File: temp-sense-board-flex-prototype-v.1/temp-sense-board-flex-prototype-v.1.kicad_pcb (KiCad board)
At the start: 2 copper layers, 134.7 x 89.8 mm, 30 parts, among them J2 FH34SRJ-12S-0.5SH(50), J3 FH12-12S-1SH(55), J4 1-84953-2, U1 TMP1075D, U2 TMP1075D, U3 TMP1075D

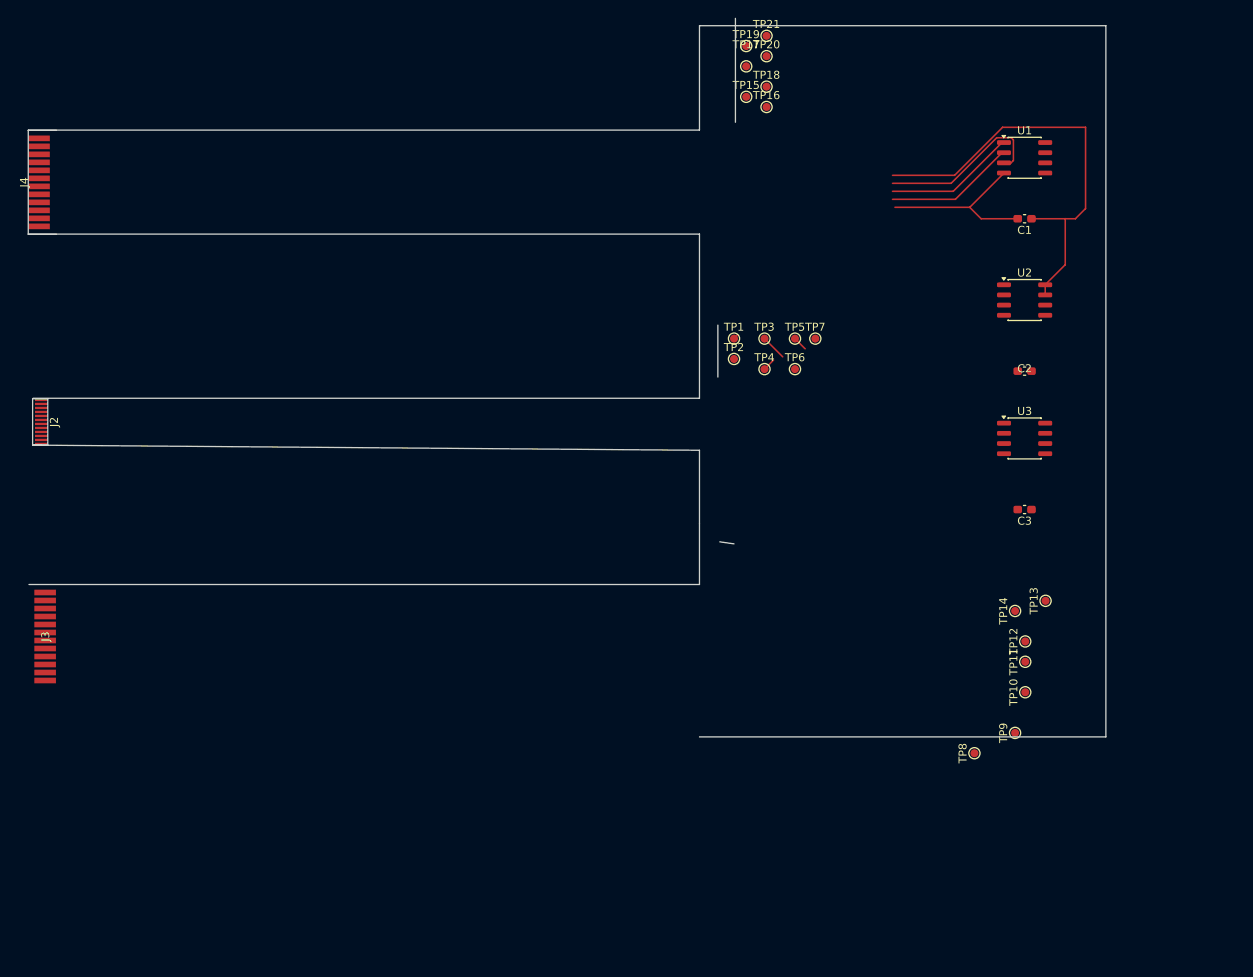
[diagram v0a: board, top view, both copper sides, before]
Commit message: outline added and layout started
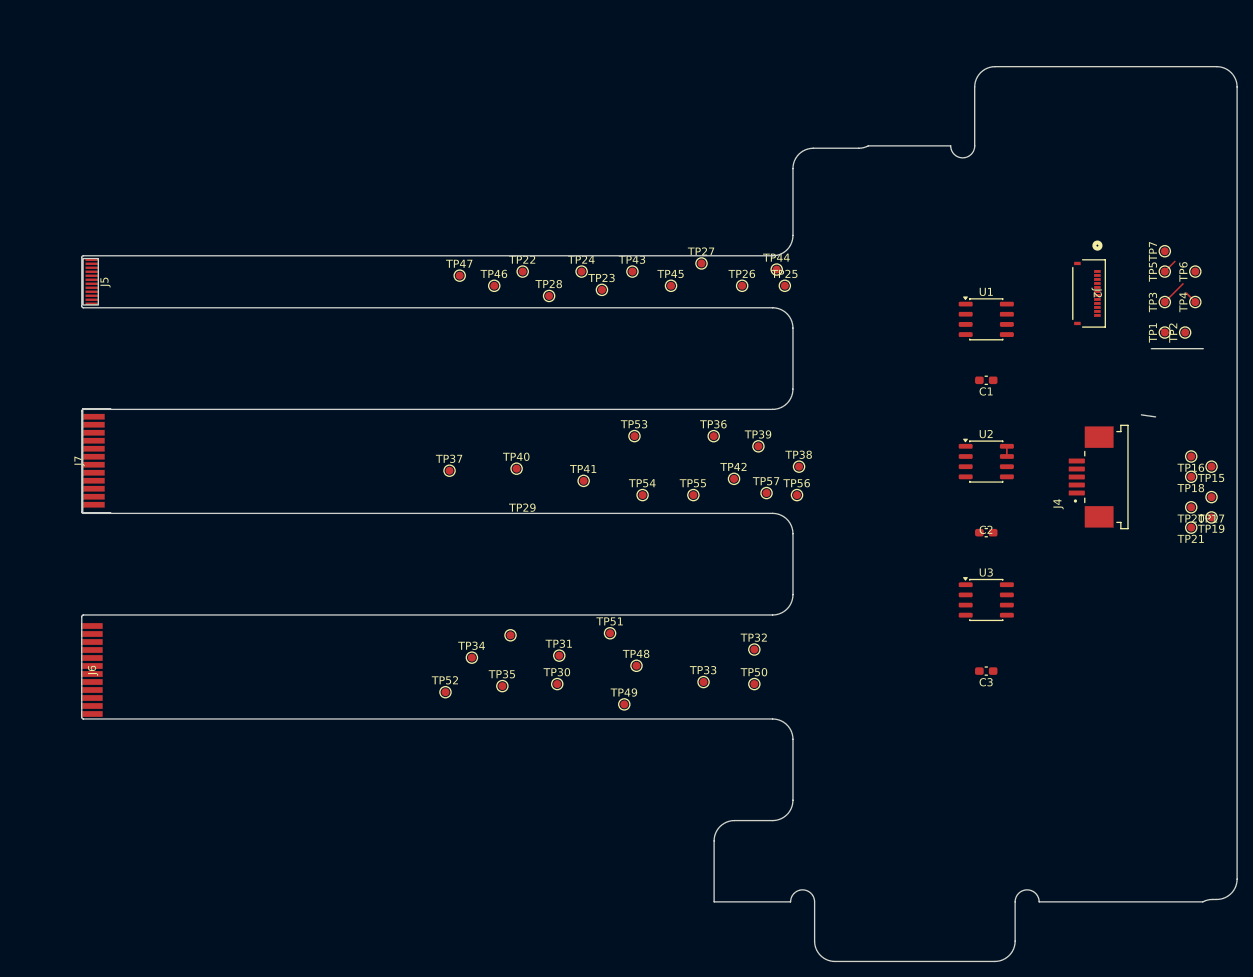
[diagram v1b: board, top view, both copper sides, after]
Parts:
- removed J3: FH12-12S-1SH(55), formula_slug_footprint_library:FPC-12PIN-CABLE-1mm-0.65mm
- removed TP10, TP11, TP12, TP13, TP14, TP8, TP9: TestPoint, TestPoint:TestPoint_Pad_D1.0mm
- added J5: FH34SRJ-12S-0.5SH(50), formula_slug_footprint_library:FPC_12-CABLE-0.5mm-0.3mm, F.Cu at (51.9, 57.4)
- added J6: FH12-12S-1SH(55), formula_slug_footprint_library:FPC-12PIN-CABLE-1mm-0.65mm, F.Cu at (49.7, 105.9)
- added J7: 1-84953-2, formula_slug_footprint_library:FPC-12PIN-CABLE-1mm-0.71mm, F.Cu at (49.9, 79.8)
- added TP22: TestPoint, TestPoint:TestPoint_Pad_D1.0mm, F.Cu at (104.9, 56.1)
- added TP23: TestPoint, TestPoint:TestPoint_Pad_D1.0mm, F.Cu at (114.8, 58.4)
- added TP24: TestPoint, TestPoint:TestPoint_Pad_D1.0mm, F.Cu at (112.3, 56.1)
- added TP25: TestPoint, TestPoint:TestPoint_Pad_D1.0mm, F.Cu at (137.7, 57.9)
- added TP26: TestPoint, TestPoint:TestPoint_Pad_D1.0mm, F.Cu at (132.3, 57.9)
- added TP27: TestPoint, TestPoint:TestPoint_Pad_D1.0mm, F.Cu at (127.3, 55.1)
- added TP28: TestPoint, TestPoint:TestPoint_Pad_D1.0mm, F.Cu at (108.2, 59.2)
- added TP29: TestPoint, TestPoint:TestPoint_Pad_D1.0mm, F.Cu at (103.4, 101.6)
- added TP30: TestPoint, TestPoint:TestPoint_Pad_D1.0mm, F.Cu at (109.2, 107.7)
- added TP31: TestPoint, TestPoint:TestPoint_Pad_D1.0mm, F.Cu at (109.5, 104.1)
- added TP32: TestPoint, TestPoint:TestPoint_Pad_D1.0mm, F.Cu at (133.9, 103.4)
- added TP33: TestPoint, TestPoint:TestPoint_Pad_D1.0mm, F.Cu at (127.5, 107.4)
- added TP34: TestPoint, TestPoint:TestPoint_Pad_D1.0mm, F.Cu at (98.6, 104.4)
- added TP35: TestPoint, TestPoint:TestPoint_Pad_D1.0mm, F.Cu at (102.4, 108.0)
- added TP36: TestPoint, TestPoint:TestPoint_Pad_D1.0mm, F.Cu at (128.8, 76.7)
- added TP37: TestPoint, TestPoint:TestPoint_Pad_D1.0mm, F.Cu at (95.8, 81.0)
- added TP38: TestPoint, TestPoint:TestPoint_Pad_D1.0mm, F.Cu at (139.4, 80.5)
- added TP39: TestPoint, TestPoint:TestPoint_Pad_D1.0mm, F.Cu at (134.4, 78.0)
- added TP40: TestPoint, TestPoint:TestPoint_Pad_D1.0mm, F.Cu at (104.1, 80.8)
- added TP41: TestPoint, TestPoint:TestPoint_Pad_D1.0mm, F.Cu at (112.5, 82.3)
- added TP42: TestPoint, TestPoint:TestPoint_Pad_D1.0mm, F.Cu at (131.3, 82.0)
- added TP43: TestPoint, TestPoint:TestPoint_Pad_D1.0mm, F.Cu at (118.6, 56.1)
- added TP44: TestPoint, TestPoint:TestPoint_Pad_D1.0mm, F.Cu at (136.7, 55.9)
- added TP45: TestPoint, TestPoint:TestPoint_Pad_D1.0mm, F.Cu at (123.4, 57.9)
- added TP46: TestPoint, TestPoint:TestPoint_Pad_D1.0mm, F.Cu at (101.3, 57.9)
- added TP47: TestPoint, TestPoint:TestPoint_Pad_D1.0mm, F.Cu at (97.0, 56.6)
- added TP48: TestPoint, TestPoint:TestPoint_Pad_D1.0mm, F.Cu at (119.1, 105.4)
- added TP49: TestPoint, TestPoint:TestPoint_Pad_D1.0mm, F.Cu at (117.6, 110.2)
- added TP50: TestPoint, TestPoint:TestPoint_Pad_D1.0mm, F.Cu at (133.9, 107.7)
- added TP51: TestPoint, TestPoint:TestPoint_Pad_D1.0mm, F.Cu at (115.8, 101.3)
- added TP52: TestPoint, TestPoint:TestPoint_Pad_D1.0mm, F.Cu at (95.2, 108.7)
- added TP53: TestPoint, TestPoint:TestPoint_Pad_D1.0mm, F.Cu at (118.9, 76.7)
- added TP54: TestPoint, TestPoint:TestPoint_Pad_D1.0mm, F.Cu at (119.9, 84.1)
- added TP55: TestPoint, TestPoint:TestPoint_Pad_D1.0mm, F.Cu at (126.2, 84.1)
- added TP56: TestPoint, TestPoint:TestPoint_Pad_D1.0mm, F.Cu at (139.2, 84.1)
- added TP57: TestPoint, TestPoint:TestPoint_Pad_D1.0mm, F.Cu at (135.4, 83.8)
- J2: footprint formula_slug_footprint_library:FPC_12-CABLE-0.5mm-0.3mm -> formula_slug_footprint_library:CONN12x1_FH34SRJ-12S-0.5SH50_HIR
- J4: footprint formula_slug_footprint_library:FPC-12PIN-CABLE-1mm-0.71mm -> formula_slug_footprint_library:TE_84952-5
- moved J4 136.1 mm to (174.2, 81.8)
- moved J2 131.1 mm to (175.7, 58.9)
- moved TP19 82.8 mm to (191.0, 86.9), turned to 180 degrees
- moved TP21 81.2 mm to (188.5, 88.1), turned to 180 degrees
- moved TP17 79.3 mm to (191.0, 84.3), turned to 180 degrees
- moved TP20 77.4 mm to (188.5, 85.6), turned to 180 degrees
- moved TP15 74.3 mm to (191.0, 80.5), turned to 180 degrees
- moved TP18 72.1 mm to (188.5, 81.8), turned to 180 degrees
- moved TP16 68.8 mm to (188.5, 79.2), turned to 180 degrees
- moved TP2 56.5 mm to (187.7, 63.8), turned to 90 degrees
- moved TP4 54.5 mm to (189.0, 59.9), turned to 90 degrees
- moved TP1 53.9 mm to (185.2, 63.8), turned to 90 degrees
- moved TP6 51.5 mm to (189.0, 56.1), turned to 90 degrees
- moved TP3 50.2 mm to (185.2, 59.9), turned to 90 degrees
- moved TP5 47.0 mm to (185.2, 56.1), turned to 90 degrees
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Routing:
- net +5V: track 54.6 -> 1.27 mm
- net V-: track 22.0 -> 0.00 mm
- net /ALERT: track 21.5 -> 0.00 mm
- net /SDA: track 16.5 -> 0.00 mm
- net /SCL: track 16.3 -> 0.00 mm
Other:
- board size 134.7 x 89.8 mm -> 144.4 x 111.8 mm
